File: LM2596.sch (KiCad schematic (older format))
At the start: 10 parts

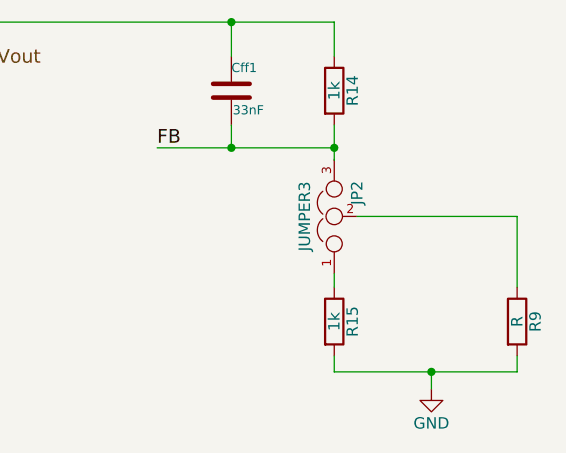
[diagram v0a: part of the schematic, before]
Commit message: Небольшие изменения
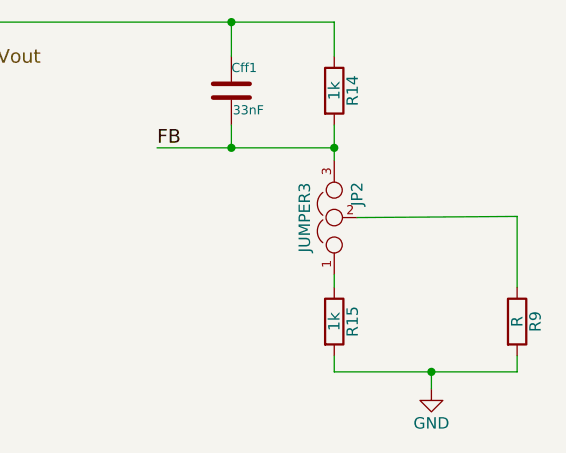
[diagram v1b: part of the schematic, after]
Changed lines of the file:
@@
 L JUMPER3 JP2
 U 1 1 5740CAA4
-P 8200 4000
-F 0 "JP2" H 8250 3900 50  0000 L CNN
-F 1 "JUMPER3" H 8200 4100 50  0000 C BNN
-F 2 "Connect:PINHEAD1-3" H 8200 4000 50  0001 C CNN
-F 3 "" H 8200 4000 50  0000 C CNN
-	1    8200 4000
+P 8200 4005
+F 0 "JP2" H 8250 3905 50  0000 L CNN
+F 1 "JUMPER3" H 8200 4105 50  0000 C BNN
+F 2 "Connect:PINHEAD1-3" H 8200 4005 50  0001 C CNN
+F 3 "" H 8200 4005 50  0000 C CNN
+	1    8200 4005
 	0    -1   -1   0
 $EndComp
@@
 Connection ~ 8200 3700
 Wire Wire Line
-	8200 4250 8200 4310
+	8200 4255 8200 4310
 Wire Wire Line
 	8200 4610 8200 4680
@@
 	9000 4310 9000 4000
 Wire Wire Line
-	9000 4000 8300 4000
+	9000 4000 8300 4005
 Wire Wire Line
 	8625 4680 8625 4755
